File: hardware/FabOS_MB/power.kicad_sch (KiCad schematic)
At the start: 22 parts, among them U501 TDPOWER TAS12-5-W2, U502 TPS563201

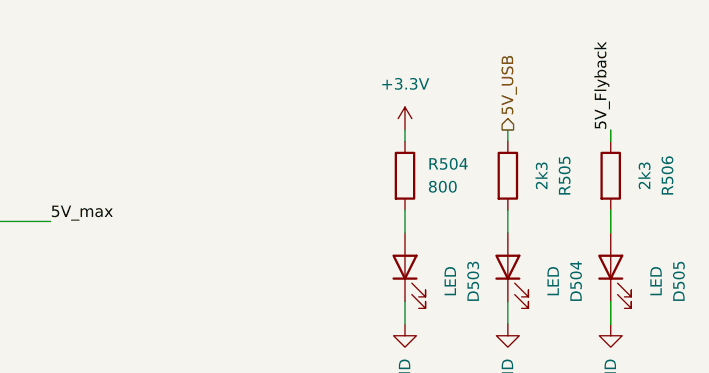
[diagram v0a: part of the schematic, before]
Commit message: connecteur programmation
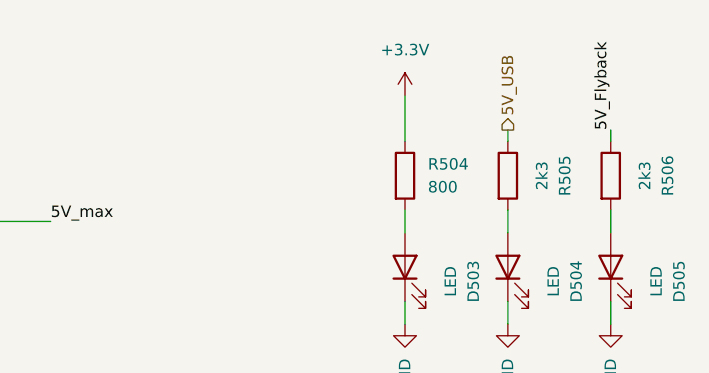
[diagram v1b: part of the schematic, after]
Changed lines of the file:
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@@
+	(wire
+		(pts
+			(xy 204.47 41.91) (xy 204.47 44.45)
+		)
+		(stroke
+			(width 0)
+			(type default)
+		)
+	)
 	(wire
 		(pts
@@
 	(wire
 		(pts
-			(xy 204.47 33.02) (xy 204.47 34.29)
-		)
-		(stroke
-			(width 0)
-			(type default)
-		)
-	)
-	(wire
-		(pts
 			(xy 220.98 120.65) (xy 220.98 119.38)
 		)
@@
 	(wire
 		(pts
-			(xy 204.47 41.91) (xy 204.47 44.45)
-		)
-		(stroke
-			(width 0)
-			(type default)
-		)
-	)
-	(wire
-		(pts
 			(xy 120.65 105.41) (xy 129.54 105.41)
 		)
@@
 		(pts
 			(xy 120.65 106.68) (xy 120.65 105.41)
+		)
+		(stroke
+			(width 0)
+			(type default)
+		)
+	)
+	(wire
+		(pts
+			(xy 204.47 29.21) (xy 204.47 34.29)
 		)
 		(stroke
@@
 	)
 	(symbol
-		(lib_id "Device:R")
-		(at 204.47 38.1 0)
-		(unit 1)
-		(exclude_from_sim no)
-		(in_bom yes)
-		(on_board yes)
-		(dnp no)
-		(fields_autoplaced yes)
-		(property "Reference" "R504"
-			(at 207.01 36.8299 0)
-			(effects
-				(font
-					(size 1.27 1.27)
-				)
-				(justify left)
-			)
-		)
-		(property "Value" "800"
-			(at 207.01 39.3699 0)
-			(effects
-				(font
-					(size 1.27 1.27)
-				)
-				(justify left)
-			)
-		)
-		(property "Footprint" ""
-			(at 202.692 38.1 90)
-			(effects
-				(font
-					(size 1.27 1.27)
-				)
-				(hide yes)
-			)
-		)
-		(property "Datasheet" "~"
-			(at 204.47 38.1 0)
-			(effects
-				(font
-					(size 1.27 1.27)
-				)
-				(hide yes)
-			)
-		)
-		(property "Description" "Resistor"
-			(at 204.47 38.1 0)
-			(effects
-				(font
-					(size 1.27 1.27)
-				)
-				(hide yes)
-			)
-		)
-		(pin "1"
-		)
-		(pin "2"
-		)
-		(instances
-			(project "FabOS_MB"
-				(path "/09377d5d-727f-4ff4-92c8-7a0483d23f1e/97fc260e-c16c-48c4-b11a-4f8ec3a451f5"
-					(reference "R504")
-					(unit 1)
-				)
-			)
-		)
-	)
-	(symbol
 		(lib_id "Jumper:SolderJumper_2_Open")
 		(at 82.55 36.83 0)
@@
 	)
 	(symbol
+		(lib_id "Device:R")
+		(at 204.47 38.1 0)
+		(unit 1)
+		(exclude_from_sim no)
+		(in_bom yes)
+		(on_board yes)
+		(dnp no)
+		(fields_autoplaced yes)
+		(property "Reference" "R504"
+			(at 207.01 36.8299 0)
+			(effects
+				(font
+					(size 1.27 1.27)
+				)
+				(justify left)
+			)
+		)
+		(property "Value" "800"
+			(at 207.01 39.3699 0)
+			(effects
+				(font
+					(size 1.27 1.27)
+				)
+				(justify left)
+			)
+		)
+		(property "Footprint" ""
+			(at 202.692 38.1 90)
+			(effects
+				(font
+					(size 1.27 1.27)
+				)
+				(hide yes)
+			)
+		)
+		(property "Datasheet" "~"
+			(at 204.47 38.1 0)
+			(effects
+				(font
+					(size 1.27 1.27)
+				)
+				(hide yes)
+			)
+		)
+		(property "Description" "Resistor"
+			(at 204.47 38.1 0)
+			(effects
+				(font
+					(size 1.27 1.27)
+				)
+				(hide yes)
+			)
+		)
+		(pin "1"
+		)
+		(pin "2"
+		)
+		(instances
+			(project "FabOS_MB"
+				(path "/09377d5d-727f-4ff4-92c8-7a0483d23f1e/97fc260e-c16c-48c4-b11a-4f8ec3a451f5"
+					(reference "R504")
+					(unit 1)
+				)
+			)
+		)
+	)
+	(symbol
 		(lib_id "Device:C_Small")
 		(at 120.65 109.22 180)
@@
 	(symbol
 		(lib_id "power:+3.3V")
-		(at 204.47 33.02 0)
+		(at 204.47 29.21 0)
 		(unit 1)
 		(exclude_from_sim no)
@@
 		(fields_autoplaced yes)
 		(property "Reference" "#PWR0512"
-			(at 204.47 36.83 0)
+			(at 204.47 33.02 0)
 			(effects
 				(font
@@
 		)
 		(property "Value" "+3.3V"
-			(at 204.47 27.94 0)
-			(effects
-				(font
-					(size 1.27 1.27)
-				)
-			)
-		)
-		(property "Footprint" ""
-			(at 204.47 33.02 0)
+			(at 204.47 24.13 0)
+			(effects
+				(font
+					(size 1.27 1.27)
+				)
+			)
+		)
+		(property "Footprint" ""
+			(at 204.47 29.21 0)
 			(effects
 				(font
@@
 		)
 		(property "Datasheet" ""
-			(at 204.47 33.02 0)
+			(at 204.47 29.21 0)
 			(effects
 				(font
@@
 		)
 		(property "Description" "Power symbol creates a global label with name \"+3.3V\""
-			(at 204.47 33.02 0)
-			(effects
-				(font
+			(at 204.47 29.21 0)
+			(effects
+				(font
